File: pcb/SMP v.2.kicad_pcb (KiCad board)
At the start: 2 copper layers, 114.7 x 58.7 mm, 36 parts, among them J1 USB_C_Receptacle_USB2.0, SW1 SW_Push, U1 ATmega32U2-AU, Y1 16MHz

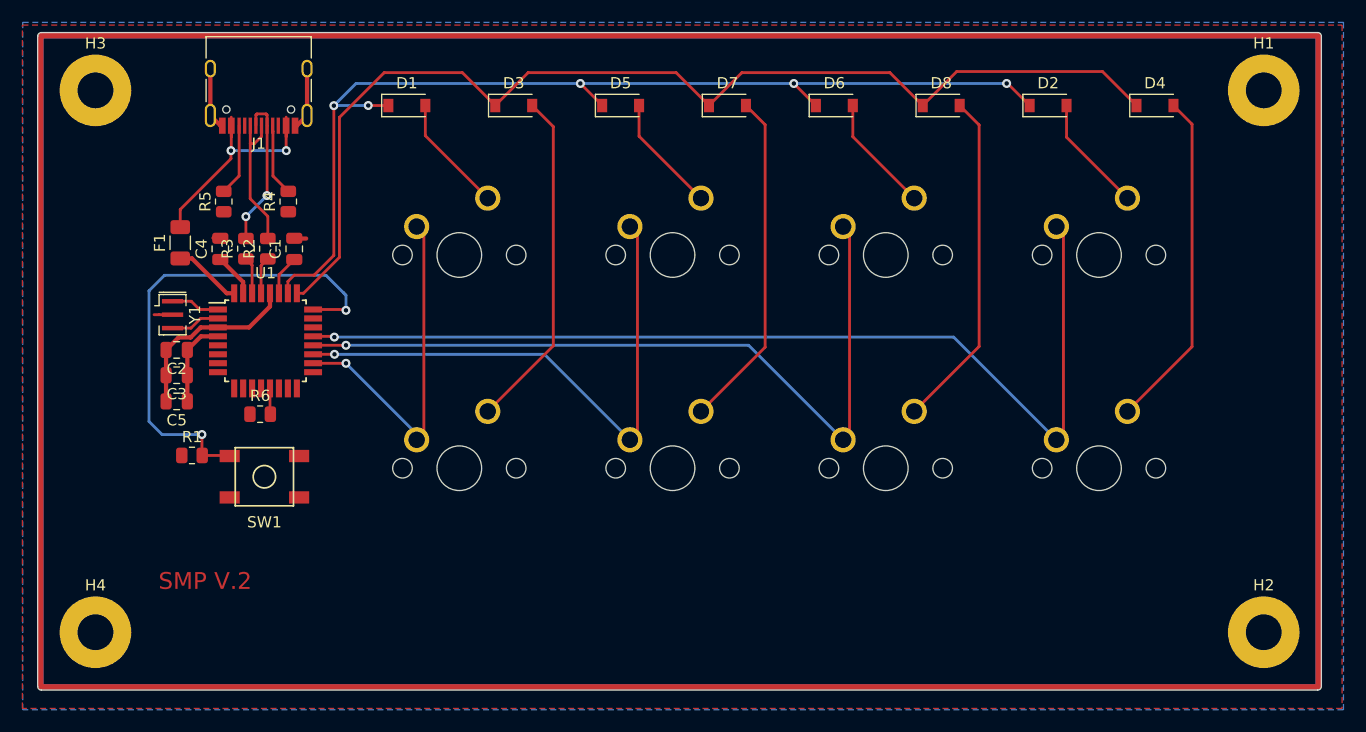
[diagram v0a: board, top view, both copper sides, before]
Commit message: latest version
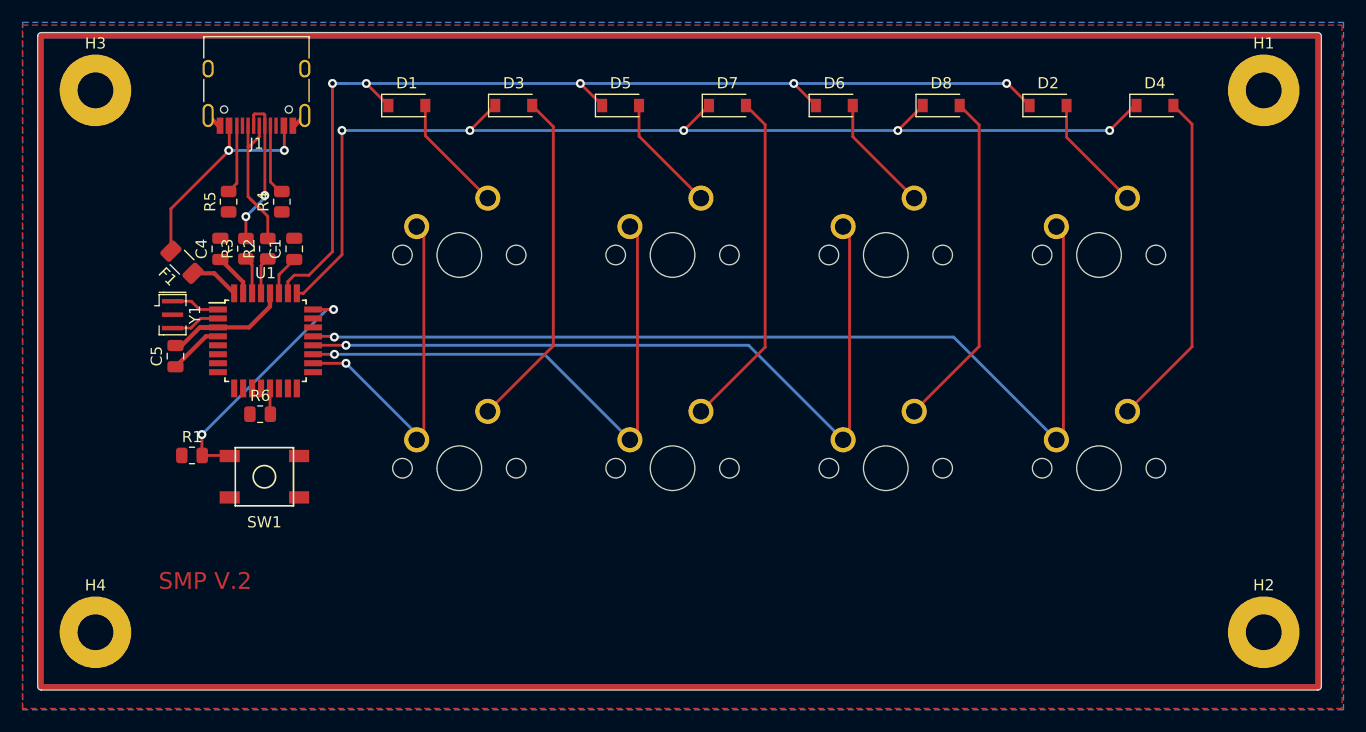
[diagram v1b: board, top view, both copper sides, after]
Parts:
- removed C2, C3: 0.1uF, Capacitor_SMD:C_0805_2012Metric
- moved C5 4.04 mm to (53.7, 54.1), turned to 90 degrees
- moved F1 1.74 mm to (54.3, 45.7), turned to 135 degrees
- moved R4 0.57 mm to (63.2, 40.3)
- moved R5 0.43 mm to (58.4, 40.3)
- moved J1 0.20 mm to (60.9, 29.5)
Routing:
- net Net-(R1-Pad2): track 44.8 -> 22.6 mm
- net GND: track 28.6 -> 15.5 mm
- net +5V: track 17.8 -> 13.2 mm
- net GNDPWR: track 1.65 -> 0.00 mm
- net Net-(F1-Pad2): track 22.2 -> 20.9 mm
- net ROW0: track 99.1 -> 98.0 mm, vias 0 -> 5
- net D+: track 13.2 -> 14.2 mm
